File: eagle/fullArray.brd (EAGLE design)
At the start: 41 x 50 mm, 96 parts

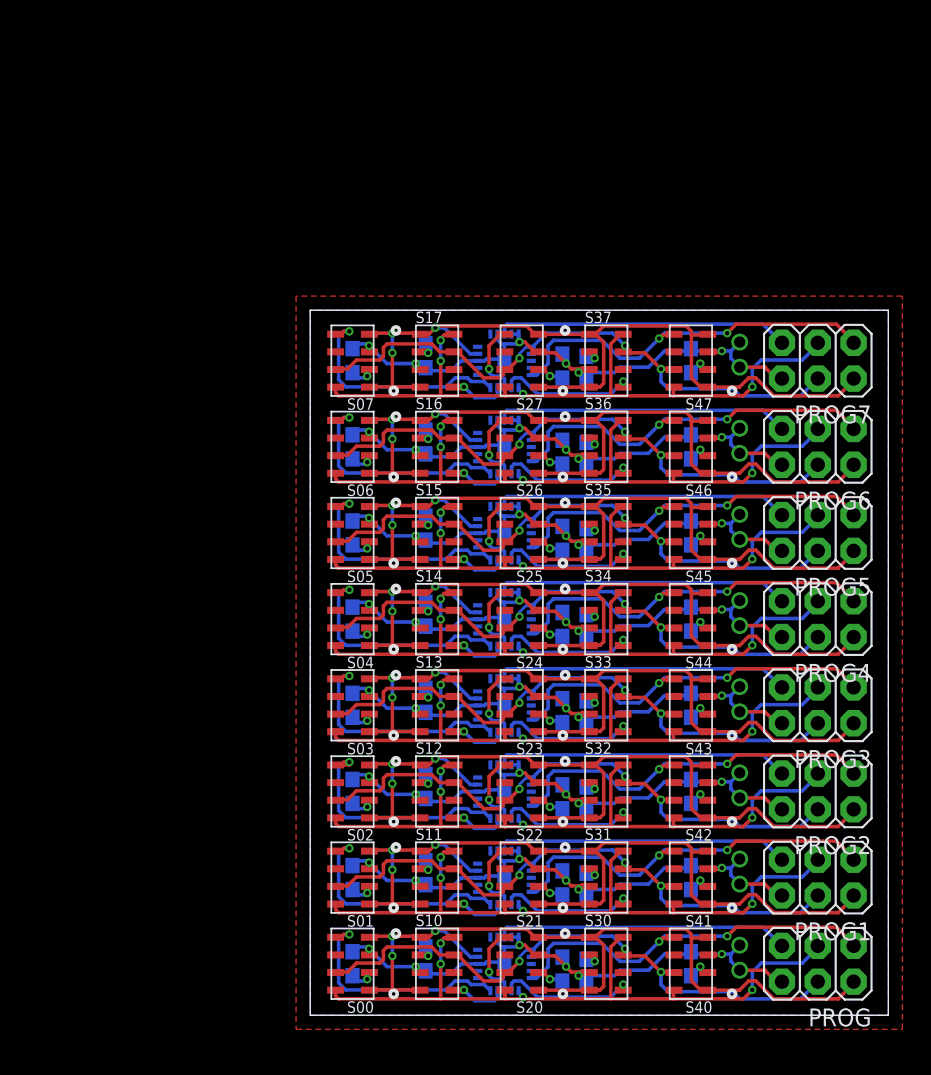
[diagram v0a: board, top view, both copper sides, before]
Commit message: Connected vertically stacked boards
Full 8-vertical layout now has power and SPI lines connected betwble een
boards.
Added the tessellatable layout go make arbitrarily high stacks.
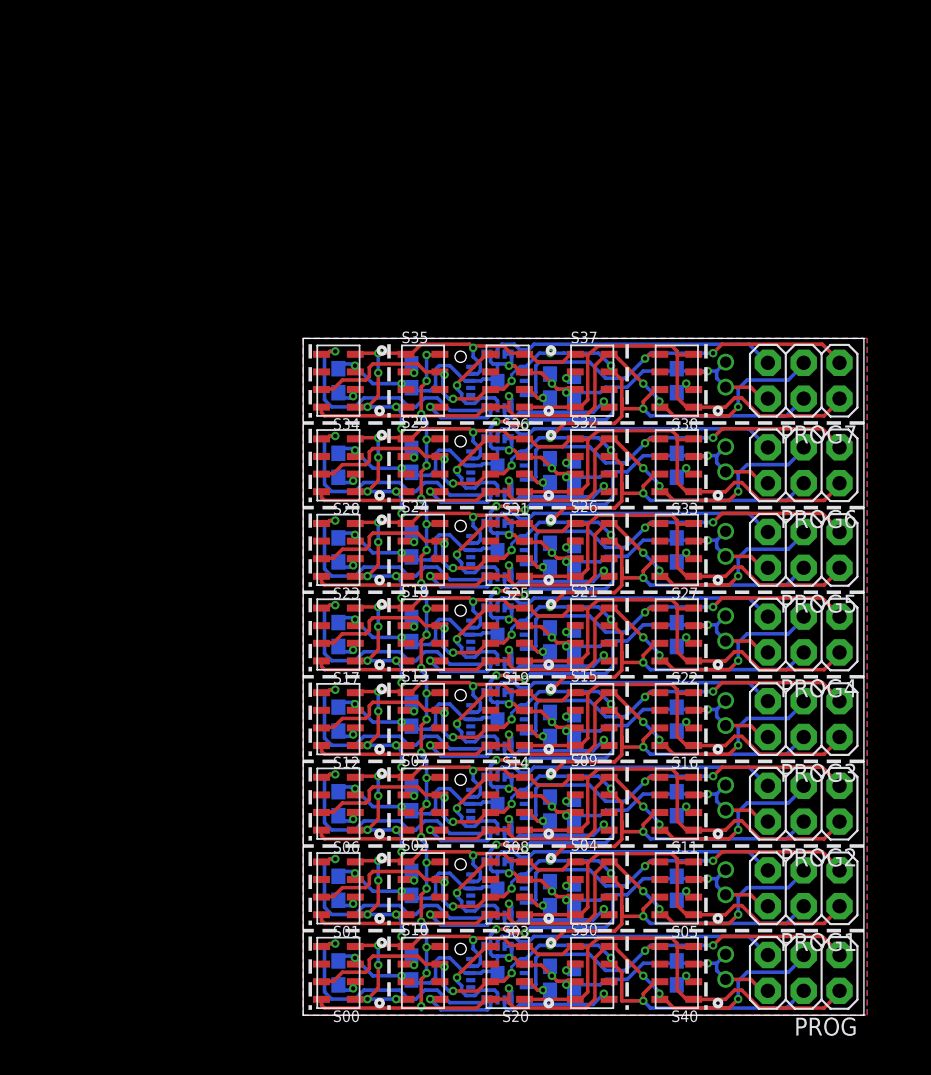
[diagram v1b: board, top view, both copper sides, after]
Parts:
- removed S41, S42, S43, S44, S45, S46, S47: MPL115A, nonolith:LGA-8
- added S08, S09, S18, S19, S28, S29, S38: MPL115A, nonolith:LGA-8
- moved S05 34.1 mm to (26.0, 9.00)
- moved S07 31.8 mm to (8.00, 15.0), turned to 0 degrees
- moved S31 30.1 mm to (14.0, 39.0), turned to 180 degrees
- moved S16 25.7 mm to (26.0, 21.0), turned to 180 degrees
- moved S04 25.6 mm to (20.0, 9.00), turned to 0 degrees
- moved S34 25.4 mm to (2.00, 45.0), turned to 180 degrees
- moved S06 25.3 mm to (2.00, 15.0)
- moved S32 23.2 mm to (20.0, 39.0)
- moved S17 20.6 mm to (2.00, 27.0), turned to 180 degrees
- moved S21 18.0 mm to (20.0, 27.0), turned to 0 degrees
- moved S11 17.8 mm to (26.0, 15.0), turned to 180 degrees
- moved S33 17.7 mm to (26.0, 39.0), turned to 180 degrees
- moved S27 17.4 mm to (26.0, 33.0)
- moved S15 17.2 mm to (20.0, 21.0)
- moved S23 17.0 mm to (2.00, 33.0)
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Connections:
- net ADDR01 renamed ADDR00-2
- net ADDR02 renamed ADDR00-3
- net ADDR03 renamed ADDR00-4
- net ADDR04 renamed ADDR00-5
- net ADDR05 renamed ADDR00-6
- net ADDR06 renamed ADDR00-7
- net ADDR07 renamed ADDR00-8
- net CAP01 renamed CAP04-2
- net CAP13 renamed CAP05-4
- net CAP25 renamed CAP01-6
- net CAP37 renamed CAP02-8
- net RESET1 renamed RESET0-2
- net RESET2 renamed RESET0-3
- net RESET3 renamed RESET0-4
- net RESET4 renamed RESET0-5
- net RESET5 renamed RESET0-6
- net RESET6 renamed RESET0-7
- net RESET7 renamed RESET0-8
- net RST01 renamed RST00-2
- net RST13 renamed RST10-4
- net RST25 renamed RST20-6
- net RST37 renamed RST30-8
- removed net CAP02: C10.1, S02.2
- removed net CAP03: C15.1, S03.2
- removed net CAP04: C20.1, S04.2
- removed net CAP05: C25.1, S05.2
- removed net CAP06: C30.1, S06.2
- removed net CAP07: C35.1, S07.2
- removed net CAP11: C6.1, S11.2
- removed net CAP12: C11.1, S12.2
- removed net CAP14: C21.1, S14.2
- removed net CAP15: C26.1, S15.2
- removed net CAP16: C31.1, S16.2
- removed net CAP17: C36.1, S17.2
- removed net CAP21: C7.1, S21.2
- removed net CAP22: C12.1, S22.2
- removed net CAP23: C17.1, S23.2
- removed net CAP24: C22.1, S24.2
- removed net CAP26: C32.1, S26.2
- removed net CAP27: C37.1, S27.2
- removed net CAP31: C8.1, S31.2
- removed net CAP32: C13.1, S32.2
- removed net CAP33: C18.1, S33.2
- removed net CAP34: C23.1, S34.2
- removed net CAP35: C28.1, S35.2
- removed net CAP36: C33.1, S36.2
- removed net CAP41: C9.1, S41.2
- removed net CAP42: C14.1, S42.2
- removed net CAP43: C19.1, S43.2
- removed net CAP44: C24.1, S44.2
- removed net CAP45: C29.1, S45.2
- removed net CAP46: C34.1, S46.2
- removed net CAP47: C39.1, S47.2
- removed net RST02: S02.5, UC2.5
- removed net RST03: S03.5, UC3.5
- removed net RST04: S04.5, UC4.5
- removed net RST05: S05.5, UC5.5
- removed net RST06: S06.5, UC6.5
- removed net RST07: S07.5, UC7.5
- removed net RST11: S11.5, UC1.4
- removed net RST12: S12.5, UC2.4
- removed net RST14: S14.5, UC4.4
- removed net RST15: S15.5, UC5.4
- removed net RST16: S16.5, UC6.4
- removed net RST17: S17.5, UC7.4
- removed net RST21: S21.5, UC1.3
- removed net RST22: S22.5, UC2.3
- removed net RST23: S23.5, UC3.3
- removed net RST24: S24.5, UC4.3
- removed net RST26: S26.5, UC6.3
- removed net RST27: S27.5, UC7.3
- removed net RST31: S31.5, UC1.2
- removed net RST32: S32.5, UC2.2
- removed net RST33: S33.5, UC3.2
- removed net RST34: S34.5, UC4.2
- removed net RST35: S35.5, UC5.2
- removed net RST36: S36.5, UC6.2
- removed net RST41: PROG1.1, S41.5, UC1.20
- removed net RST42: PROG2.1, S42.5, UC2.20
- removed net RST43: PROG3.1, S43.5, UC3.20
- removed net RST44: PROG4.1, S44.5, UC4.20
- removed net RST45: PROG5.1, S45.5, UC5.20
- removed net RST46: PROG6.1, S46.5, UC6.20
- removed net RST47: PROG7.1, S47.5, UC7.20
- new net CAP01-2: C7.1, S03.2
- new net CAP01-3: C12.1, S08.2
- new net CAP01-4: C17.1, S14.2
- new net CAP01-5: C22.1, S19.2
- new net CAP01-7: C32.1, S31.2
- new net CAP01-8: C37.1, S36.2
- new net CAP02-2: C8.1, S04.2
- new net CAP02-3: C13.1, S09.2
- new net CAP02-4: C18.1, S15.2
- new net CAP02-5: C23.1, S21.2
- new net CAP02-6: C28.1, S26.2
- new net CAP02-7: C33.1, S32.2
- new net CAP03-2: C9.1, S05.2
- new net CAP03-3: C14.1, S11.2
- new net CAP03-4: C19.1, S16.2
- new net CAP03-5: C24.1, S22.2
- new net CAP03-6: C29.1, S27.2
- new net CAP03-7: C34.1, S33.2
- new net CAP03-8: C39.1, S38.2
- new net CAP04-3: C10.1, S06.2
- new net CAP04-4: C15.1, S12.2
- new net CAP04-5: C20.1, S17.2
- new net CAP04-6: C25.1, S23.2
- new net CAP04-7: C30.1, S28.2
- new net CAP04-8: C35.1, S34.2
- new net CAP05-2: C6.1, S02.2
- new net CAP05-3: C11.1, S07.2
- new net CAP05-5: C21.1, S18.2
- new net CAP05-6: C26.1, S24.2
- new net CAP05-7: C31.1, S29.2
- new net CAP05-8: C36.1, S35.2
- new net RST00-3: S06.5, UC2.5
- new net RST00-4: S12.5, UC3.5
- new net RST00-5: S17.5, UC4.5
- new net RST00-6: S23.5, UC5.5
- new net RST00-7: S28.5, UC6.5
- new net RST00-8: S34.5, UC7.5
- new net RST10-2: S02.5, UC1.4
- new net RST10-3: S07.5, UC2.4
- new net RST10-5: S18.5, UC4.4
- new net RST10-6: S24.5, UC5.4
- new net RST10-7: S29.5, UC6.4
- new net RST10-8: S35.5, UC7.4
- new net RST20-2: S03.5, UC1.3
- new net RST20-3: S08.5, UC2.3
- new net RST20-4: S14.5, UC3.3
- new net RST20-5: S19.5, UC4.3
- new net RST20-7: S31.5, UC6.3
- new net RST20-8: S36.5, UC7.3
- new net RST30-2: S04.5, UC1.2
- new net RST30-3: S09.5, UC2.2
- new net RST30-4: S15.5, UC3.2
- new net RST30-5: S21.5, UC4.2
- new net RST30-6: S26.5, UC5.2
- new net RST30-7: S32.5, UC6.2
- new net RST40-2: PROG1.1, S05.5, UC1.20
- new net RST40-3: PROG2.1, S11.5, UC2.20
- new net RST40-4: PROG3.1, S16.5, UC3.20
- new net RST40-5: PROG4.1, S22.5, UC4.20
- new net RST40-6: PROG5.1, S27.5, UC5.20
- new net RST40-7: PROG6.1, S33.5, UC6.20
- new net RST40-8: PROG7.1, S38.5, UC7.20
- net 3.3V: now also S08.1, S08.4, S09.1, S09.4, S18.1, S18.4, S19.1, S19.4, S28.1, S28.4, S29.1, S29.4, S38.1, S38.4; no longer S41.1, S41.4, S42.1, S42.4, S43.1, S43.4, S44.1, S44.4, S45.1, S45.4, S46.1, S46.4, S47.1, S47.4
- net GND: now also S08.3, S09.3, S18.3, S19.3, S28.3, S29.3, S38.3; no longer S41.3, S42.3, S43.3, S44.3, S45.3, S46.3, S47.3
- net SCL: now also S08.8, S09.8, S18.8, S19.8, S28.8, S29.8, S38.8; no longer S41.8, S42.8, S43.8, S44.8, S45.8, S46.8, S47.8
- net SDA: now also S08.7, S09.7, S18.7, S19.7, S28.7, S29.7, S38.7; no longer S41.7, S42.7, S43.7, S44.7, S45.7, S46.7, S47.7
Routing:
- net GND: track 384.4 -> 482.9 mm, vias 64 -> 78
- net SDA: track 345.5 -> 415.9 mm, vias 24 -> 48
- net SCL: track 403.7 -> 433.8 mm, vias 32 -> 56
- net RST47: track 27.9 -> 0.00 mm, vias 2 -> 0
- net RST46: track 27.9 -> 0.00 mm, vias 2 -> 0
- net RST45: track 27.9 -> 0.00 mm, vias 2 -> 0
- net RST44: track 27.9 -> 0.00 mm, vias 2 -> 0
- net RST43: track 27.9 -> 0.00 mm, vias 2 -> 0
- net RST42: track 27.9 -> 0.00 mm, vias 2 -> 0
- net RST40-8: track 0.00 -> 27.7 mm, vias 0 -> 2
- net RST40-7: track 0.00 -> 27.7 mm, vias 0 -> 2
- net RST40-6: track 0.00 -> 27.7 mm, vias 0 -> 2
- net RST40-5: track 0.00 -> 27.7 mm, vias 0 -> 2
- net RST40-4: track 0.00 -> 27.7 mm, vias 0 -> 2
- net RST40-3: track 0.00 -> 27.7 mm, vias 0 -> 2
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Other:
- board size 41 x 50 mm -> 39.8 x 48 mm

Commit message: added four row board w/ USB interface.
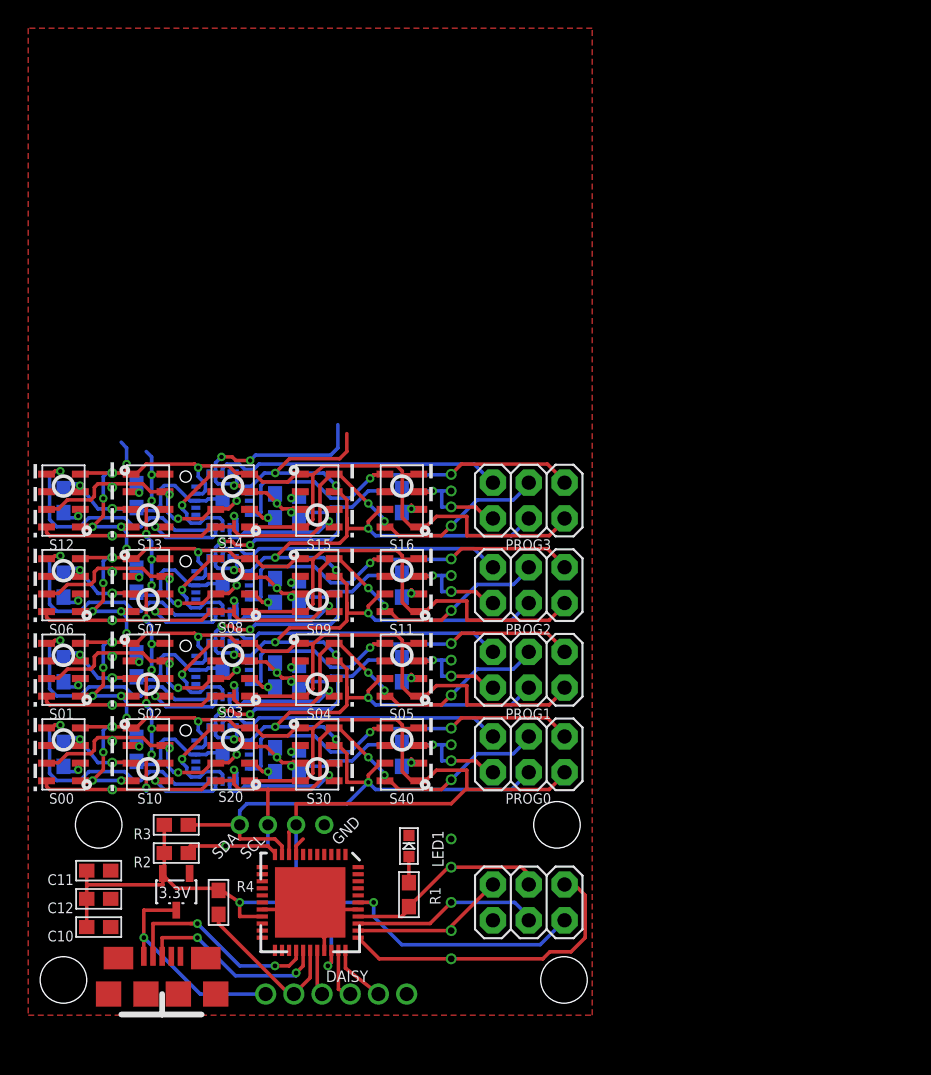
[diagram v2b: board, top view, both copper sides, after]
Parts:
- removed C23, C24, C25, C26, C27, C28, C29, C30, C31, C32, C33, C34, C35, C36, C37, C38, C39: (no value), nonolith:0603
- removed PROG4, PROG5, PROG6, PROG7: (no value), nonolith:2X03
- removed S17, S18, S19, S21, S22, S23, S24, S25, S26, S27, S28, S29, S31, S32, S33, S34, S35, S36, S37, S38: MPL115A, nonolith:LGA-8
- removed UC4, UC5, UC6, UC7: ATTINY24QFN, nonolith:QFN20
- added 3.3V: VREG, nonolith:SOT23-3
- added CN1: (no value), nonolith:USB-MICROB
- added DAISY: (no value), nonolith:1X06_ROUND_2MM
- added IC1: (no value), nonolith:QFN-44
- added JP1, JP2, SCL, SDA: (no value), nonolith:1X01_2MM
- added LED1: (no value), microbuilder:CHIPLED_0603
- added PROG0: (no value), nonolith:2X03
- added R1, R2, R3, R4: (no value), nonolith:0603
- added U$1, U$2, U$3, U$4: (no value), nonolith:STAND-OFF
- C10: value (none) -> 1uF
- C11: value (none) -> .1uF
- C12: value (none) -> .01uF
- moved C14 41.5 mm to (-12.3, 30.9), turned to 270 degrees
- moved C19 41.5 mm to (-12.3, 36.9), turned to 270 degrees
- moved C13 39.6 mm to (-17.5, 30.5), turned to 90 degrees
- moved C18 39.6 mm to (-17.5, 36.5), turned to 90 degrees
- moved C12 32.6 mm to (-15.0, 8.25), flipped to the top, turned to 180 degrees
- moved C0 24.9 mm to (-17.5, 18.5)
- moved C1 24.9 mm to (-12.3, 18.9)
- moved C2 24.9 mm to (-2.49, 18.1)
- moved C3 24.9 mm to (-0.78, 18.0)
- moved C4 24.9 mm to (6.50, 18.5)
- moved C5 24.9 mm to (-17.5, 24.5)
- moved C6 24.9 mm to (-12.3, 24.9)
- moved C7 24.9 mm to (-2.49, 24.1)
- moved C8 24.9 mm to (-0.78, 24.0)
- moved C9 24.9 mm to (6.50, 24.5)
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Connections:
- net ADDR00-2 renamed ADDR01
- net ADDR00-3 renamed ADDR02
- net ADDR00-4 renamed ADDR03
- net CAP01-2 renamed CAP01
- net CAP02-2 renamed CAP02
- net CAP03-2 renamed CAP03
- net CAP04-2 renamed CAP04
- net CAP05-2 renamed CAP05
- net RESET0-2 renamed RESET1
- net RESET0-3 renamed RESET2
- net RESET0-4 renamed RESET3
- net RST00-2 renamed RST01
- net RST00-3 renamed RST02
- net RST00-4 renamed RST03
- net RST10-2 renamed RST11
- net RST10-3 renamed RST12
- net RST10-4 renamed RST13
- net RST20-2 renamed RST21
- net RST20-3 renamed RST22
- net RST20-4 renamed RST23
- net RST30-2 renamed RST31
- net RST30-3 renamed RST32
- net RST30-4 renamed RST33
- net RST40-2 renamed RST41
- net RST40-3 renamed RST42
- net RST40-4 renamed RST43
- removed net ADDR00-5: UC4.11
- removed net ADDR00-6: UC5.11
- removed net ADDR00-7: UC6.11
- removed net ADDR00-8: UC7.11
- removed net CAP01-3: C12.1, S08.2
- removed net CAP01-4: C17.1, S14.2
- removed net CAP01-5: C22.1, S19.2
- removed net CAP01-6: C27.1, S25.2
- removed net CAP01-7: C32.1, S31.2
- removed net CAP01-8: C37.1, S36.2
- removed net CAP02-3: C13.1, S09.2
- removed net CAP02-4: C18.1, S15.2
- removed net CAP02-5: C23.1, S21.2
- removed net CAP02-6: C28.1, S26.2
- removed net CAP02-7: C33.1, S32.2
- removed net CAP02-8: C38.1, S37.2
- removed net CAP03-3: C14.1, S11.2
- removed net CAP03-4: C19.1, S16.2
- removed net CAP03-5: C24.1, S22.2
- removed net CAP03-6: C29.1, S27.2
- removed net CAP03-7: C34.1, S33.2
- removed net CAP03-8: C39.1, S38.2
- removed net CAP04-3: C10.1, S06.2
- removed net CAP04-4: C15.1, S12.2
- removed net CAP04-5: C20.1, S17.2
- removed net CAP04-6: C25.1, S23.2
- removed net CAP04-7: C30.1, S28.2
- removed net CAP04-8: C35.1, S34.2
- removed net CAP05-3: C11.1, S07.2
- removed net CAP05-4: C16.1, S13.2
- removed net CAP05-5: C21.1, S18.2
- removed net CAP05-6: C26.1, S24.2
- removed net CAP05-7: C31.1, S29.2
- removed net CAP05-8: C36.1, S35.2
- removed net RESET0-5: PROG4.5, UC4.13
- removed net RESET0-6: PROG5.5, UC5.13
- removed net RESET0-7: PROG6.5, UC6.13
- removed net RESET0-8: PROG7.5, UC7.13
- removed net RST00-5: S17.5, UC4.5
- removed net RST00-6: S23.5, UC5.5
- removed net RST00-7: S28.5, UC6.5
- removed net RST00-8: S34.5, UC7.5
- removed net RST10-5: S18.5, UC4.4
- removed net RST10-6: S24.5, UC5.4
- removed net RST10-7: S29.5, UC6.4
- removed net RST10-8: S35.5, UC7.4
- removed net RST20-5: S19.5, UC4.3
- removed net RST20-6: S25.5, UC5.3
- removed net RST20-7: S31.5, UC6.3
- removed net RST20-8: S36.5, UC7.3
- removed net RST30-5: S21.5, UC4.2
- removed net RST30-6: S26.5, UC5.2
- removed net RST30-7: S32.5, UC6.2
- removed net RST30-8: S37.5, UC7.2
- removed net RST40-5: PROG4.1, S22.5, UC4.20
- removed net RST40-6: PROG5.1, S27.5, UC5.20
- removed net RST40-7: PROG6.1, S33.5, UC6.20
- removed net RST40-8: PROG7.1, S38.5, UC7.20
- new net 5V: 3.3V.3, CN1.P1, DAISY.6
- new net BOOTLOAD: IC1.36, PROG.4
- new net CAP06: C15.1, S08.2
- new net CAP07: C16.1, S09.2
- new net CAP08: C17.1, S11.2
- new net CAP09: C13.1, S06.2
- new net CAP11: C14.1, S07.2
- new net CAP12: C20.1, S14.2
- new net CAP13: C21.1, S15.2
- new net CAP14: C22.1, S16.2
- new net CAP15: C18.1, S12.2
- new net CAP16: C19.1, S13.2
- new net PDI-CLK: IC1.35, PROG.5
- new net PDI-DATA: IC1.34, PROG.1
- new net PE0: DAISY.5, IC1.28, R4.1
- new net PE1: DAISY.4, IC1.29
- new net PE2: DAISY.3, IC1.32
- new net PE3: DAISY.2, IC1.33
- new net PR1: IC1.37, PROG.3, R1.1
- new net PR1-P: LED1.A, R1.2
- new net USB+: CN1.P3, IC1.27
- new net USB-: CN1.P2, IC1.26
- net 3.3V: now also 3.3V.2, C10.2, C11.2, C12.2, IC1.19, IC1.31, IC1.39, IC1.9, JP2.1, PROG0.2, R2.2, R3.2, R4.2; no longer PROG4.2, PROG5.2, PROG6.2, PROG7.2, S17.1, S17.4, S18.1, S18.4, S19.1, S19.4, S21.1, S21.4, S22.1, S22.4, S23.1, S23.4, S24.1, S24.4, S25.1, S25.4, S26.1, S26.4, S27.1, S27.4, S28.1, S28.4, S29.1, S29.4, S31.1, S31.4, S32.1, S32.4, S33.1, S33.4, S34.1, S34.4, S35.1, S35.4, S36.1, S36.4, S37.1, S37.4, S38.1, S38.4, UC4.9, UC5.9, UC6.9, UC7.9
- net GND: now also 3.3V.1, C10.1, C11.1, C12.1, CN1.P5, DAISY.1, IC1.18, IC1.30, IC1.38, IC1.8, JP1.1, LED1.C, PROG0.6; no longer C10.2, C11.2, C12.2, C23.2, C24.2, C25.2, C26.2, C27.2, C28.2, C29.2, C30.2, C31.2, C32.2, C33.2, C34.2, C35.2, C36.2, C37.2, C38.2, C39.2, PROG4.6, PROG5.6, PROG6.6, PROG7.6, S17.3, S18.3, S19.3, S21.3, S22.3, S23.3, S24.3, S25.3, S26.3, S27.3, S28.3, S29.3, S31.3, S32.3, S33.3, S34.3, S35.3, S36.3, S37.3, S38.3, UC4.0, UC4.12, UC4.14, UC4.15, UC4.8, UC5.0, UC5.12, UC5.14, UC5.15, UC5.8, UC6.0, UC6.12, UC6.14, UC6.15, UC6.8, UC7.0, UC7.12, UC7.14, UC7.15, UC7.8
- net RESET0: now also PROG0.5; no longer PROG.5
- net RST40: now also PROG0.1; no longer PROG.1
- net SCL: now also IC1.11, PROG0.3, R2.1, SCL.1; no longer PROG.3, PROG4.3, PROG5.3, PROG6.3, PROG7.3, S17.8, S18.8, S19.8, S21.8, S22.8, S23.8, S24.8, S25.8, S26.8, S27.8, S28.8, S29.8, S31.8, S32.8, S33.8, S34.8, S35.8, S36.8, S37.8, S38.8, UC4.1, UC5.1, UC6.1, UC7.1
- net SDA: now also IC1.10, PROG0.4, R3.1, SDA.1; no longer PROG.4, PROG4.4, PROG5.4, PROG6.4, PROG7.4, S17.7, S18.7, S19.7, S21.7, S22.7, S23.7, S24.7, S25.7, S26.7, S27.7, S28.7, S29.7, S31.7, S32.7, S33.7, S34.7, S35.7, S36.7, S37.7, S38.7, UC4.16, UC5.16, UC6.16, UC7.16
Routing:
- net GND: track 482.9 -> 262.7 mm, vias 78 -> 40
- net SCL: track 433.8 -> 228.8 mm, vias 56 -> 33
- net SDA: track 415.9 -> 231.9 mm, vias 48 -> 28
- net 3.3V: track 512.7 -> 340.4 mm, vias 47 -> 27
- net RST40-8: track 27.7 -> 0.00 mm, vias 2 -> 0
- net RST40-7: track 27.7 -> 0.00 mm, vias 2 -> 0
- net RST40-6: track 27.7 -> 0.00 mm, vias 2 -> 0
- net RST40-5: track 27.7 -> 0.00 mm, vias 2 -> 0
- net PDI-DATA: track 0.00 -> 22.1 mm
- net RESET0-5: track 20.6 -> 0.00 mm
- net RESET0-8: track 20.6 -> 0.00 mm
- net RESET0-7: track 20.6 -> 0.00 mm
- net RESET0-6: track 20.6 -> 0.00 mm
- net RST00-6: track 18.0 -> 0.00 mm, vias 1 -> 0
- net RST00-5: track 18.0 -> 0.00 mm, vias 1 -> 0
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- removed copper zone on layer 16, net GND
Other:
- board outline removed
- board text added: "C"
- board text added: "D"
- board text added: "G"
- board text added: "GND"
- board text added: "SCL"
- board text added: "SDA"
- board text added: "V"
